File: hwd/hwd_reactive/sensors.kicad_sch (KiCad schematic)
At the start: 22 parts

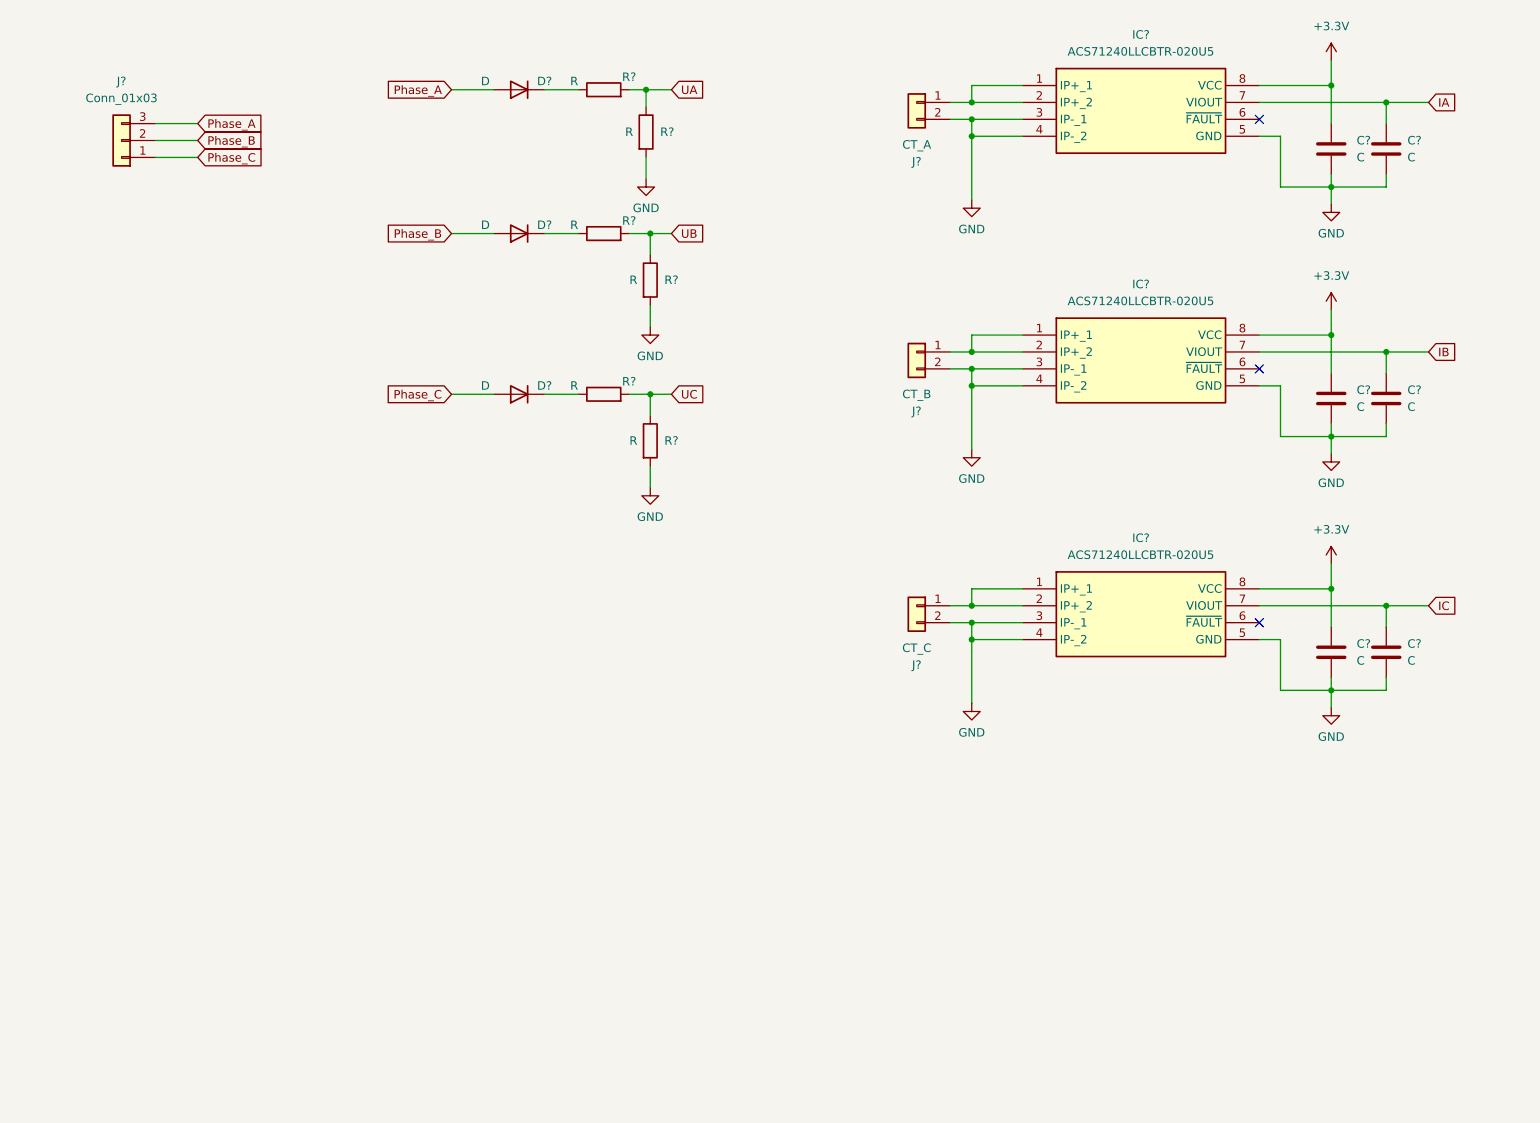
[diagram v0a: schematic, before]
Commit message: added code for testing
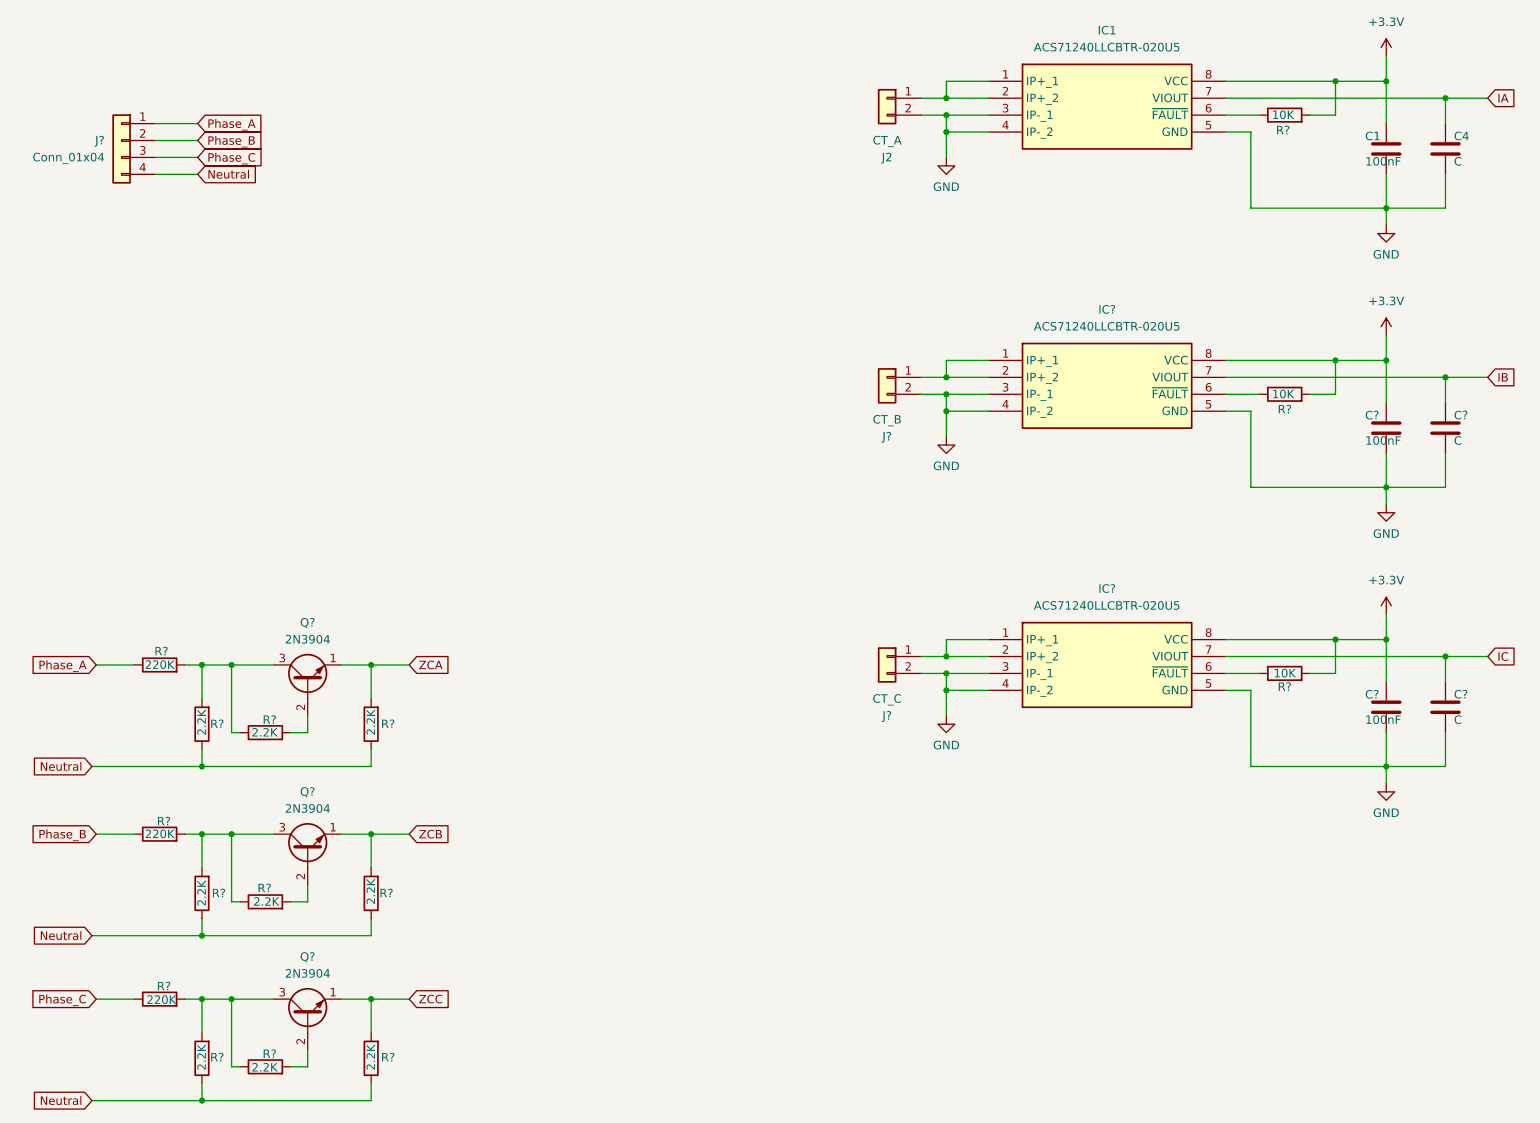
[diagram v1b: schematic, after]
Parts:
- removed C? (x4): C, symbol Device:C
- removed D? (x3): D, symbol Device:D
- removed IC? (x2): ACS71240LLCBTR-020U5, SOIC127P600X175-8N, symbol acs712:ACS71240LLCBTR-020U5
- removed J?: CT_B, symbol Connector_Generic:Conn_01x02
- removed J?: CT_C, symbol Connector_Generic:Conn_01x02
- removed J?: Conn_01x03, symbol Connector_Generic:Conn_01x03
- removed R? (x6): R, symbol Device:R
- added C? (x2): 100nF, symbol Device:C
- added C? (x2): C, symbol Device:C
- added IC? (x2): ACS71240LLCBTR-020U5, SOIC127P600X175-8N, symbol acs712:ACS71240LLCBTR-020U5
- added J?: Conn_01x04, symbol Connector_Generic:Conn_01x04
- added J?: CT_C, symbol Connector_Generic:Conn_01x02
- added J?: CT_B, symbol Connector_Generic:Conn_01x02
- added Q? (x3): 2N3904, Package_TO_SOT_THT:TO-92_Inline, symbol Transistor_BJT:2N3904
- added R? (x9): 2.2K, symbol Device:R
- added R? (x3): 10K, symbol Device:R
- added R? (x3): 220K, symbol Device:R
- C1: renamed from C?; value C -> 100nF
- gave numbers to parts that had none: 3
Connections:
- net +3.3V: now also C?.1, C?.1, IC?.8 (VCC), IC?.8 (VCC), R?.2, R?.2, R?.2
- net GND: now also C?.2, C?.2, C?.2, C?.2, IC?.3 (IP-_1), IC?.3 (IP-_1), IC?.4 (IP-_2), IC?.4 (IP-_2), IC?.5 (GND), IC?.5 (GND), J?.2 (Pin_2), J?.2 (Pin_2)
- net IB: now also C?.1, IC?.7 (VIOUT)
- net IC: now also C?.1, IC?.7 (VIOUT)
- net Phase_A: now also J?.1 (Pin_1), R?.1
- net Phase_B: now also J?.2 (Pin_2), R?.1
- net Phase_C: now also J?.3 (Pin_3), R?.1
- net at IC1.6 (~{FAULT}): now also R?.1
- new net: Q?.3 (C), R?.1, R?.2, R?.2 (x3)
- new net: Q?.2 (B), R?.2 (x3)
- new net: IC?.1 (IP+_1), IC?.2 (IP+_2), J?.1 (Pin_1) (x2)
- new net: IC?.6 (~{FAULT}), R?.1 (x2)
- new net Neutral: J?.4 (Pin_4), R?.1, R?.1, R?.1, R?.1, R?.1, R?.1
- new net ZCA: Q?.1 (E), R?.2
- new net ZCB: Q?.1 (E), R?.2
- new net ZCC: Q?.1 (E), R?.2
- no-connect marks 3 -> 0
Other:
- moved on the sheet: C1, C4, IC1, J2
